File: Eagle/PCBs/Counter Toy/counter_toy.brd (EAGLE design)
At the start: 55.9 x 81.3 mm, 210 parts, among them Q100 2N7002, Q101 2N7002, Q102 2N7002, Q103 2N7002, Q104 2N7002, Q105 2N7002, Q106 2N7002, Q11 2N7002, Q12 2N7002, Q126 2N7002, Q127 2N7002, Q128 2N7002, Q129 2N7002, Q130 2N7002, Q131 2N7002, Q132 2N7002, Q133 2N7002, Q134 2N7002, Q135 2N7002, Q136 2N7002, Q137 2N7002, Q138 2N7002, Q139 2N7002, Q140 2N7002, Q141 2N7002, Q142 2N7002, Q162 2N7002, Q163 2N7002, Q164 2N7002, Q165 2N7002, Q166 2N7002, Q167 2N7002, Q168 2N7002, Q169 2N7002, Q170 2N7002, Q171 2N7002, Q172 2N7002, Q173 2N7002, Q174 2N7002, Q175 2N7002, Q176 2N7002, Q177 2N7002, Q178 2N7002, Q18 2N7002, Q19 2N7002, Q198 2N7002, Q199 2N7002, Q2 2N7002, Q20 2N7002, Q200 2N7002, Q201 2N7002, Q202 2N7002, Q203 2N7002, Q204 2N7002, Q205 2N7002, Q206 2N7002, Q207 2N7002, Q208 2N7002, Q209 2N7002, Q210 2N7002, Q211 2N7002, Q212 2N7002, Q213 2N7002, Q214 2N7002, Q24 2N7002, Q25 2N7002, Q26 2N7002, Q27 2N7002, Q28 2N7002, Q29 2N7002, Q30 2N7002, Q31 2N7002, Q32 2N7002, Q33 2N7002, Q34 2N7002, Q36 2N7002, Q37 2N7002, Q38 2N7002, Q39 2N7002, Q40 2N7002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

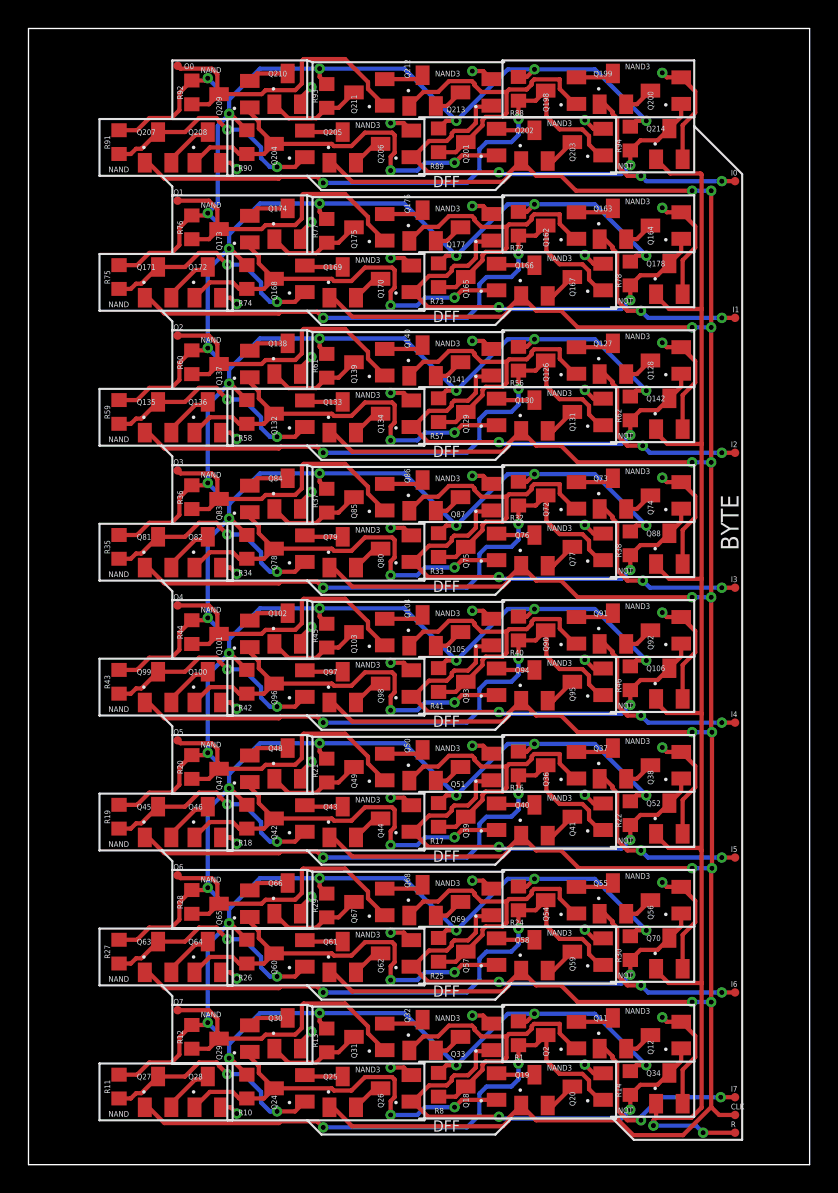
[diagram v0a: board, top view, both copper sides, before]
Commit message: Update counter_toy.brd
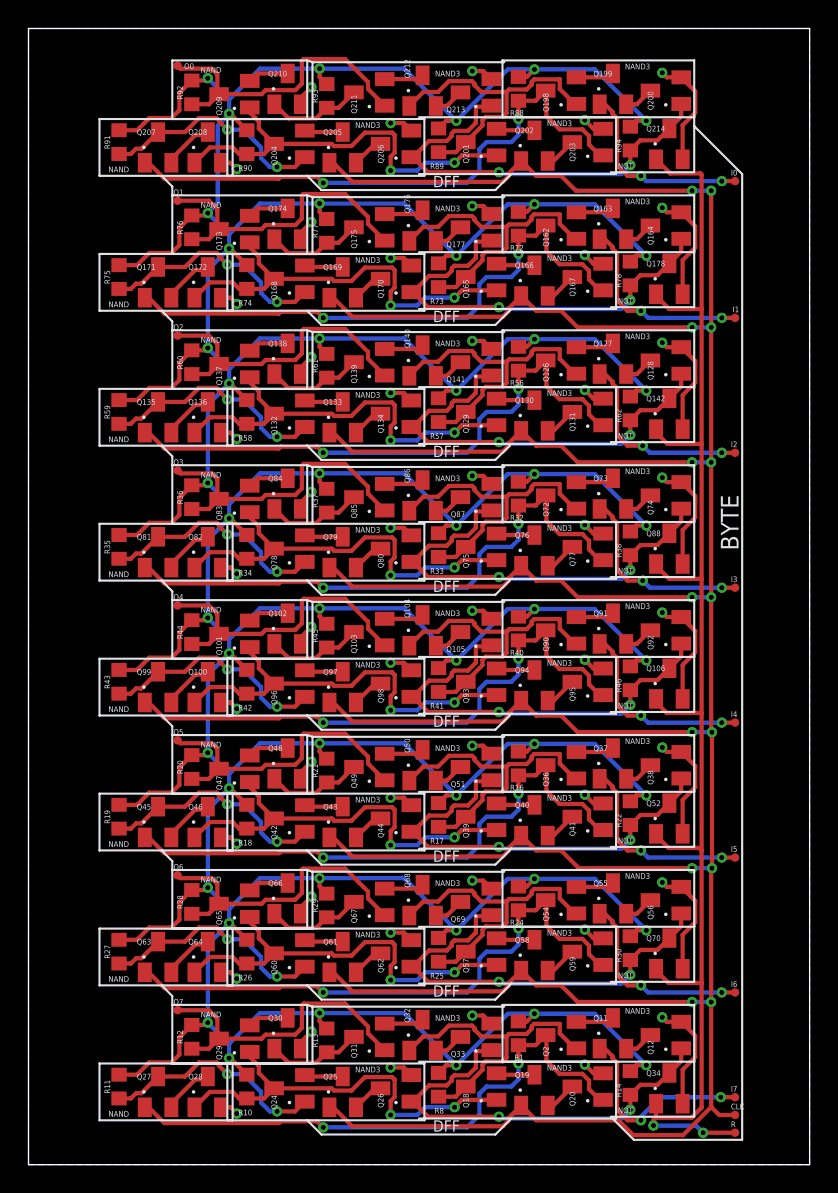
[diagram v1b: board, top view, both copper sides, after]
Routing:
- added copper zone on layer 16, net GND
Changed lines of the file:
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@@
 </layers>
 <board>
-<fusionsync huburn="a.cGVyc29uYWw6dWUyZGY0M2Ex" projecturn="a.cGVyc29uYWw6dWUyZGY0M2ExIzIwMjEwMTIwMzczOTE5OTMx" f3durn="urn:adsk.wipprod:dm.lineage:RKQa1e1pTIef6ifPqg5Tig" pcbguid="" lastpulledtime="" lastsyncedchangeguid="" latestrevisionid="468e08d1-bdf0-40c3-9270-53415b291e36" lastsyncedrevisionid="468e08d1-bdf0-40c3-9270-53415b291e36" lastboardhashguid="1fa0f9e9-e586-e5ba-25a4-847b196b3b5a" lastpushedtime="2023-04-18T12:42:12Z" linktopcb3d="true"/>
+<fusionsync huburn="a.cGVyc29uYWw6dWUyZGY0M2Ex" projecturn="a.cGVyc29uYWw6dWUyZGY0M2ExIzIwMjEwMTIwMzczOTE5OTMx" f3durn="urn:adsk.wipprod:dm.lineage:RKQa1e1pTIef6ifPqg5Tig" pcbguid="" lastpulledtime="" lastsyncedchangeguid="" latestrevisionid="ae0b7da3-c6b2-42a1-a777-f11f63b34cd7" lastsyncedrevisionid="ae0b7da3-c6b2-42a1-a777-f11f63b34cd7" lastboardhashguid="42e16079-18b1-1462-3737-b46bbdbd1827" lastpushedtime="2023-04-19T04:21:05Z" linktopcb3d="true"/>
 <plain>
 <wire x1="33.909" y1="11.43" x2="47.625" y2="11.43" width="0.1524" layer="21"/>
@@
 <wire x1="40.4249625" y1="74.102" x2="39.7995625" y2="74.7274" width="0.3048" layer="1"/>
 <via x="39.7995625" y="74.7274" extent="1-16" drill="0.35"/>
-<wire x1="45.339" y1="68.453" x2="46.797" y2="71.925" width="0" layer="19" extent="1-1"/>
-<wire x1="45.339" y1="58.801" x2="46.797" y2="62.273" width="0" layer="19" extent="1-1"/>
-<wire x1="45.339" y1="49.149" x2="46.797" y2="52.621" width="0" layer="19" extent="1-1"/>
-<wire x1="45.339" y1="39.497" x2="46.797" y2="42.969" width="0" layer="19" extent="1-1"/>
-<wire x1="45.339" y1="29.845" x2="46.797" y2="33.317" width="0" layer="19" extent="1-1"/>
-<wire x1="45.339" y1="20.193" x2="46.797" y2="23.665" width="0" layer="19" extent="1-1"/>
-<wire x1="45.339" y1="10.541" x2="46.797" y2="14.013" width="0" layer="19" extent="1-1"/>
-<wire x1="41.105" y1="74.102" x2="45.339" y2="78.105" width="0" layer="19" extent="1-1"/>
-<wire x1="41.105" y1="64.45" x2="45.339" y2="68.453" width="0" layer="19" extent="1-1"/>
-<wire x1="41.105" y1="54.798" x2="45.339" y2="58.801" width="0" layer="19" extent="1-1"/>
-<wire x1="41.105" y1="45.146" x2="45.339" y2="49.149" width="0" layer="19" extent="1-1"/>
-<wire x1="41.105" y1="35.494" x2="45.339" y2="39.497" width="0" layer="19" extent="1-1"/>
-<wire x1="41.105" y1="25.842" x2="45.339" y2="29.845" width="0" layer="19" extent="1-1"/>
-<wire x1="41.105" y1="16.19" x2="45.339" y2="20.193" width="0" layer="19" extent="1-1"/>
-<wire x1="41.105" y1="6.538" x2="45.339" y2="10.541" width="0" layer="19" extent="1-1"/>
-<wire x1="33.104" y1="77.658" x2="39.7995625" y2="74.7274" width="0" layer="19" extent="1-1"/>
-<wire x1="27.389" y1="73.975" x2="31.75" y2="78.232" width="0" layer="19" extent="1-1"/>
-<wire x1="20.241" y1="77.089" x2="25.908" y2="74.5128" width="0" layer="19" extent="1-1"/>
-<wire x1="14.90041875" y1="71.2222" x2="19.492" y2="75.862" width="0" layer="19" extent="1-1"/>
-<wire x1="20.241" y1="67.437" x2="14.90041875" y2="71.2222" width="0" layer="19" extent="1-1"/>
-<wire x1="25.908" y1="64.8608" x2="20.241" y2="67.437" width="0" layer="19" extent="1-1"/>
-<wire x1="31.75" y1="68.58" x2="27.389" y2="64.323" width="0" layer="19" extent="1-1"/>
-<wire x1="14.90041875" y1="61.5702" x2="19.492" y2="66.21" width="0" layer="19" extent="1-1"/>
-<wire x1="20.241" y1="57.785" x2="14.90041875" y2="61.5702" width="0" layer="19" extent="1-1"/>
-<wire x1="25.908" y1="55.2088" x2="20.241" y2="57.785" width="0" layer="19" extent="1-1"/>
-<wire x1="31.75" y1="58.928" x2="27.389" y2="54.671" width="0" layer="19" extent="1-1"/>
-<wire x1="14.90041875" y1="51.9182" x2="19.492" y2="56.558" width="0" layer="19" extent="1-1"/>
-<wire x1="20.241" y1="48.133" x2="14.90041875" y2="51.9182" width="0" layer="19" extent="1-1"/>
-<wire x1="25.908" y1="45.5568" x2="20.241" y2="48.133" width="0" layer="19" extent="1-1"/>
-<wire x1="31.75" y1="49.276" x2="27.389" y2="45.019" width="0" layer="19" extent="1-1"/>
-<wire x1="14.90041875" y1="42.2662" x2="19.492" y2="46.906" width="0" layer="19" extent="1-1"/>
-<wire x1="20.241" y1="38.481" x2="14.90041875" y2="42.2662" width="0" layer="19" extent="1-1"/>
-<wire x1="25.908" y1="35.9048" x2="20.241" y2="38.481" width="0" layer="19" extent="1-1"/>
-<wire x1="31.75" y1="39.624" x2="27.389" y2="35.367" width="0" layer="19" extent="1-1"/>
-<wire x1="14.90041875" y1="32.6142" x2="19.492" y2="37.254" width="0" layer="19" extent="1-1"/>
-<wire x1="20.241" y1="28.829" x2="14.90041875" y2="32.6142" width="0" layer="19" extent="1-1"/>
-<wire x1="25.908" y1="26.2528" x2="20.241" y2="28.829" width="0" layer="19" extent="1-1"/>
-<wire x1="31.75" y1="29.972" x2="27.389" y2="25.715" width="0" layer="19" extent="1-1"/>
-<wire x1="14.90041875" y1="22.9622" x2="19.492" y2="27.602" width="0" layer="19" extent="1-1"/>
-<wire x1="20.241" y1="19.177" x2="14.90041875" y2="22.9622" width="0" layer="19" extent="1-1"/>
-<wire x1="25.908" y1="16.6008" x2="20.241" y2="19.177" width="0" layer="19" extent="1-1"/>
-<wire x1="31.75" y1="20.32" x2="27.389" y2="16.063" width="0" layer="19" extent="1-1"/>
-<wire x1="14.90041875" y1="13.3102" x2="19.492" y2="17.95" width="0" layer="19" extent="1-1"/>
-<wire x1="20.241" y1="9.525" x2="14.90041875" y2="13.3102" width="0" layer="19" extent="1-1"/>
-<wire x1="25.908" y1="6.9488" x2="20.241" y2="9.525" width="0" layer="19" extent="1-1"/>
-<wire x1="31.75" y1="10.668" x2="27.389" y2="6.411" width="0" layer="19" extent="1-1"/>
-<wire x1="14.90041875" y1="3.6582" x2="19.492" y2="8.298" width="0" layer="19" extent="1-1"/>
+<polygon width="0.0762" layer="16">
+<vertex x="0" y="0"/>
+<vertex x="55.88" y="0"/>
+<vertex x="55.88" y="81.28"/>
+<vertex x="0" y="81.28"/>
+</polygon>
 </signal>
 <signal name="N$11">
